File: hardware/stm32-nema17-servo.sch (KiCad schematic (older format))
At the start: 91 parts, among them J1 Conn_01x05, J2 C31-S-RA-CS1A-BK-SS, J3 TC-2050, J4 Screw_Terminal_01x02, J5 Screw_Terminal_01x02, J7 Conn_01x03, J8 Conn_01x03, J9 Conn_01x02, M1 Stepper_Motor_bipolar, Q1 NTTFS4937N, Q10 SSM3K35CTC, Q2 NVTFS5C658NL, Q3 NVTFS5C658NL, Q4 NVTFS5C658NL, Q5 NVTFS5C658NL, Q6 NVTFS5C658NL, Q7 NVTFS5C658NL, Q8 SSM3K35CTC, Q9 SSM3K35CTC, SW1 EVP-BB2A9B000, U1 STM32G431CBU, U2 74LVC2G32, U3 UCC27516, U4 AS5047D, U5 TPS62172DSG, U6 DRV8323RS

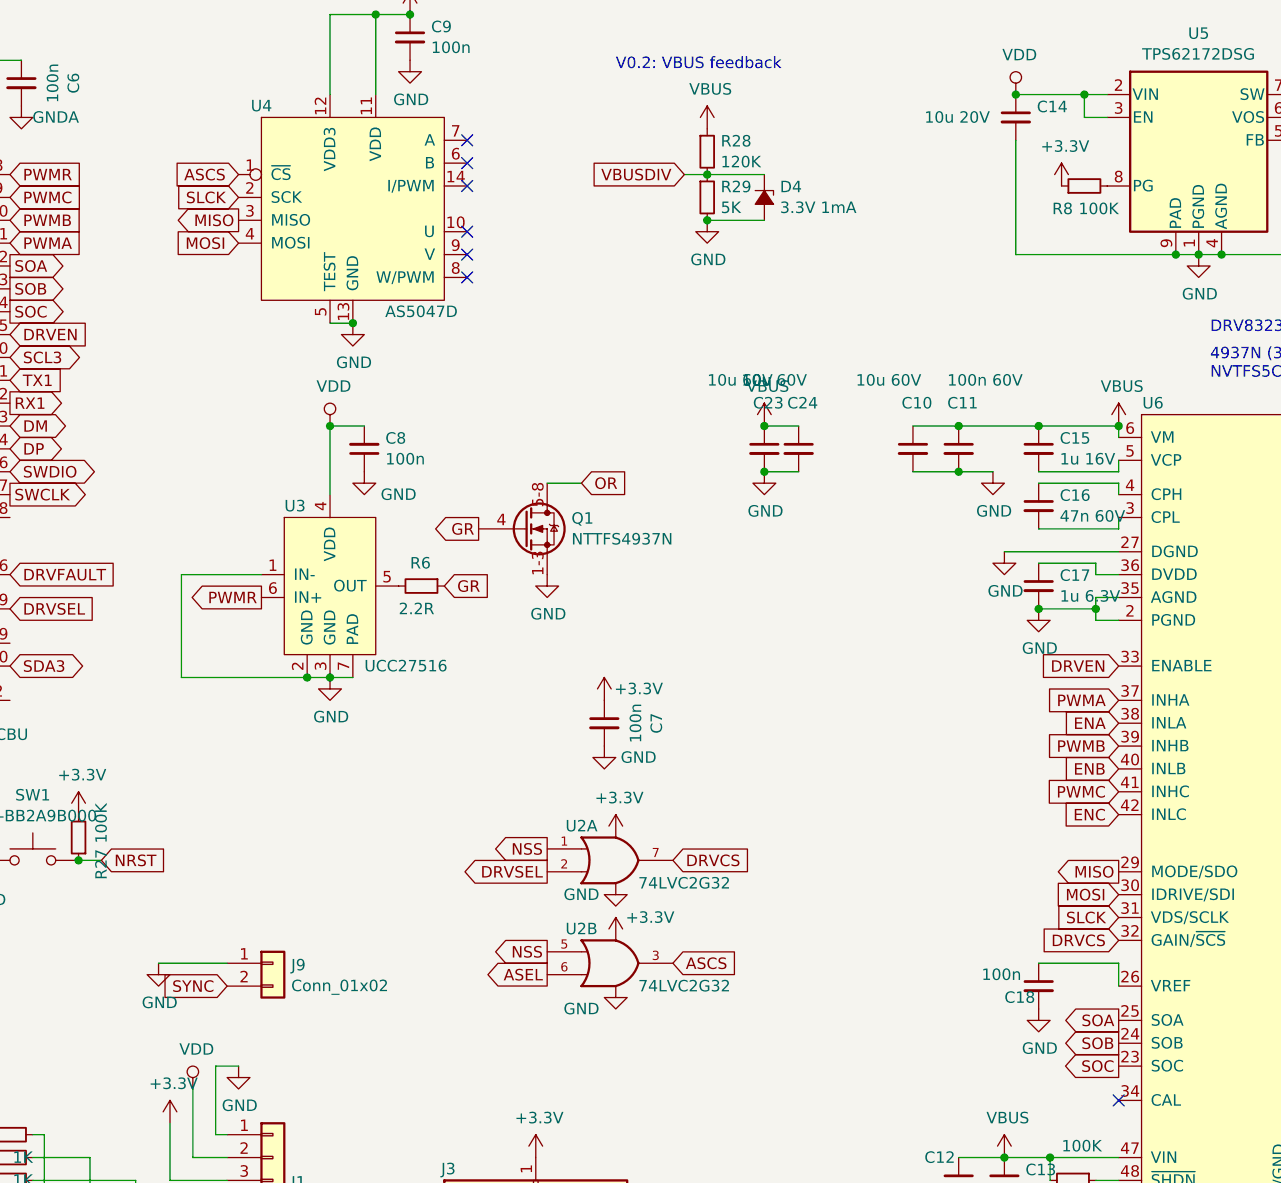
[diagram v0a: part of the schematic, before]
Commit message: further fixes on v0.2 hardware
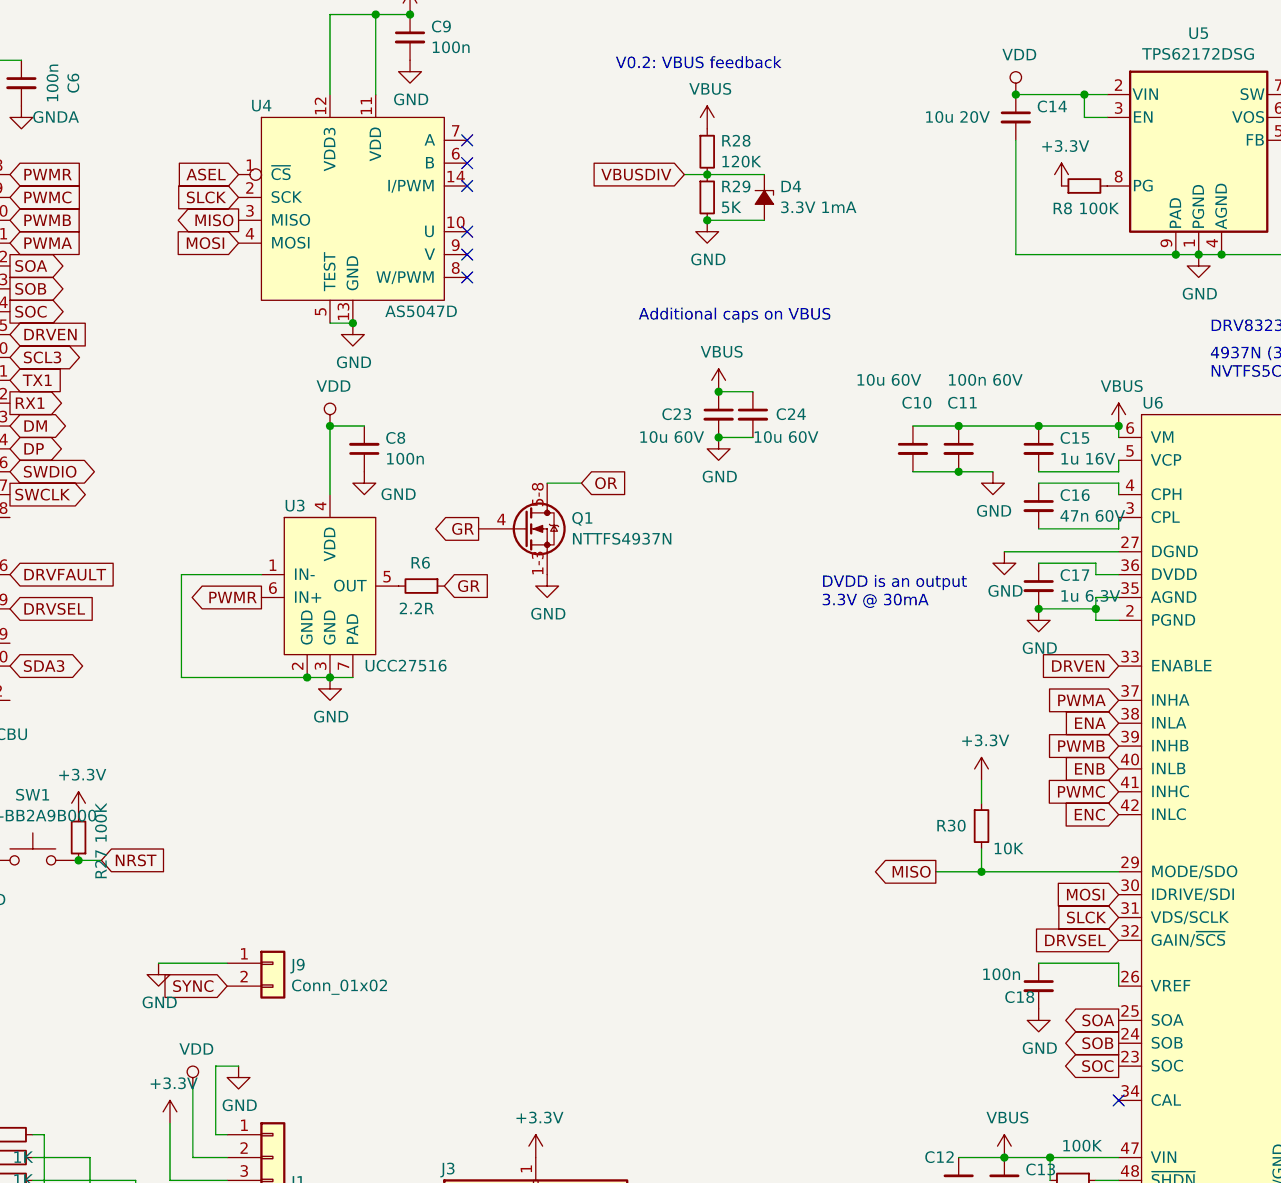
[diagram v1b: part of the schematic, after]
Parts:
- removed C7: 100n, Capacitor_SMD:C_0402_1005Metric, symbol Device:C_Small
- removed U2: 74LVC2G32, Package_SON:X2SON-8_1.4x1mm_P0.35mm, symbol 74xGxx:74LVC2G32
- added R30: 10K, Resistor_SMD:R_0402_1005Metric, symbol Device:R_Small
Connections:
- net ASCS is gone; now on net ASEL: U4.1 (~CS)
- net DRVCS is gone; now on net DRVSEL: U6.32 (GAIN/~SCS)
- net +3V3: now also R30.1
- net MISO: now also R30.2
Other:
- note added: "Additional caps on VBUS"
- note added: "DVDD is an output\n3.3V @ 30mA"
- moved on the sheet: C23, C24
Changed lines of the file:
@@
 Text GLabel 7450 4400 0    50   Input ~ 0
 ENC
-Text GLabel 7450 4650 0    50   Output ~ 0
+Text GLabel 6650 4650 0    50   Output ~ 0
 MISO
 Text GLabel 7450 4750 0    50   Input ~ 0
@@
 SLCK
 Text GLabel 7450 4950 0    50   Input ~ 0
-DRVCS
+DRVSEL
 Text GLabel 3600 1600 0    50   Input ~ 0
-ASCS
+ASEL
 Text GLabel 2600 1900 2    50   Input ~ 0
 PWMA
@@
 Text GLabel 1300 3700 0    50   Input ~ 0
 SLCK
-Text GLabel 5500 5050 2    50   Input ~ 0
-ASCS
-Text GLabel 5500 4600 2    50   Input ~ 0
-DRVCS
 Text GLabel 7450 5300 0    50   Output ~ 0
 SOA
@@
 	3150 6300 3550 6300
 Connection ~ 3150 6300
-Text GLabel 4950 4650 0    50   Output ~ 0
-DRVSEL
-Text GLabel 4950 5100 0    50   Output ~ 0
-ASEL
 Text GLabel 2600 3500 2    50   Input ~ 0
 DRVSEL
@@
 L Device:C_Small C23
 U 1 1 5D56448D
-P 5900 2800
-F 0 "C23" H 5850 3000 50  0000 L CNN
-F 1 "10u 60V" H 5650 3100 50  0000 L CNN
-F 2 "Capacitor_SMD:C_1210_3225Metric" H 5900 2800 50  0001 C CNN
-F 3 "~" H 5900 2800 50  0001 C CNN
-	1    5900 2800
+P 5700 2650
+F 0 "C23" H 5450 2650 50  0000 L CNN
+F 1 "10u 60V" H 5350 2550 50  0000 L CNN
+F 2 "Capacitor_SMD:C_1210_3225Metric" H 5700 2650 50  0001 C CNN
+F 3 "~" H 5700 2650 50  0001 C CNN
+	1    5700 2650
 	1    0    0    -1
 $EndComp
@@
 L power:VBUS #PWR059
 U 1 1 5D567754
-P 5900 2700
-F 0 "#PWR059" H 5900 2550 50  0001 C CNN
-F 1 "VBUS" H 5915 2873 50  0000 C CNN
-F 2 "" H 5900 2700 50  0001 C CNN
-F 3 "" H 5900 2700 50  0001 C CNN
-	1    5900 2700
+P 5700 2550
+F 0 "#PWR059" H 5700 2400 50  0001 C CNN
+F 1 "VBUS" H 5715 2723 50  0000 C CNN
+F 2 "" H 5700 2550 50  0001 C CNN
+F 3 "" H 5700 2550 50  0001 C CNN
+	1    5700 2550
 	1    0    0    -1
 $EndComp
@@
 L power:GND #PWR060
 U 1 1 5D56F0C9
-P 5900 2900
-F 0 "#PWR060" H 5900 2650 50  0001 C CNN
-F 1 "GND" H 5905 2727 50  0000 C CNN
-F 2 "" H 5900 2900 50  0001 C CNN
-F 3 "" H 5900 2900 50  0001 C CNN
-	1    5900 2900
+P 5700 2750
+F 0 "#PWR060" H 5700 2500 50  0001 C CNN
+F 1 "GND" H 5705 2577 50  0000 C CNN
+F 2 "" H 5700 2750 50  0001 C CNN
+F 3 "" H 5700 2750 50  0001 C CNN
+	1    5700 2750
 	1    0    0    -1
 $EndComp
@@
 L Device:C_Small C24
 U 1 1 5D57E91C
-P 6050 2800
-F 0 "C24" H 6000 3000 50  0000 L CNN
-F 1 "10u 60V" H 5800 3100 50  0000 L CNN
-F 2 "Capacitor_SMD:C_1210_3225Metric" H 6050 2800 50  0001 C CNN
-F 3 "~" H 6050 2800 50  0001 C CNN
-	1    6050 2800
-	1    0    0    -1
-$EndComp
-Wire Wire Line
-	5900 2700 6050 2700
-Connection ~ 5900 2700
-Wire Wire Line
-	6050 2900 5900 2900
-Connection ~ 5900 2900
+P 5850 2650
+F 0 "C24" H 5950 2650 50  0000 L CNN
+F 1 "10u 60V" H 5850 2550 50  0000 L CNN
+F 2 "Capacitor_SMD:C_1210_3225Metric" H 5850 2650 50  0001 C CNN
+F 3 "~" H 5850 2650 50  0001 C CNN
+	1    5850 2650
+	1    0    0    -1
+$EndComp
+Wire Wire Line
+	5700 2550 5850 2550
+Connection ~ 5700 2550
+Wire Wire Line
+	5850 2750 5700 2750
+Connection ~ 5700 2750
 $Comp
 L Switch:SW_Push SW1
@@
 Text Notes 5250 1150 0    50   ~ 0
 V0.2: VBUS feedback
-$Comp
-L power:GND #PWR017
-U 1 1 5D97ADCA
-P 5200 4100
-F 0 "#PWR017" H 5200 3850 50  0001 C CNN
-F 1 "GND" H 5350 4050 50  0000 C CNN
-F 2 "" H 5200 4100 50  0001 C CNN
-F 3 "" H 5200 4100 50  0001 C CNN
-	1    5200 4100
+Text Notes 6150 3500 0    50   ~ 0
+DVDD is an output\n3.3V @ 30mA
+Text Notes 5350 2250 0    50   ~ 0
+Additional caps on VBUS
+$Comp
+L Device:R_Small R30
+U 1 1 5D7DCDEC
+P 6850 4450
+F 0 "R30" H 6650 4450 50  0000 L CNN
+F 1 "10K" H 6900 4350 50  0000 L CNN
+F 2 "Resistor_SMD:R_0402_1005Metric" H 6850 4450 50  0001 C CNN
+F 3 "~" H 6850 4450 50  0001 C CNN
+	1    6850 4450
 	1    0    0    -1
 $EndComp
 $Comp
 L power:+3.3V #PWR016
-U 1 1 5D97AAED
-P 5200 3900
-F 0 "#PWR016" H 5200 3750 50  0001 C CNN
-F 1 "+3.3V" H 5350 3950 50  0000 C CNN
-F 2 "" H 5200 3900 50  0001 C CNN
-F 3 "" H 5200 3900 50  0001 C CNN
-	1    5200 3900
-	1    0    0    -1
-$EndComp
-$Comp
-L Device:C_Small C7
-U 1 1 5D97A3CE
-P 5200 4000
-F 0 "C7" V 5429 4000 50  0000 C CNN
-F 1 "100n" V 5338 4000 50  0000 C CNN
-F 2 "Capacitor_SMD:C_0402_1005Metric" H 5200 4000 50  0001 C CNN
-F 3 "~" H 5200 4000 50  0001 C CNN
-	1    5200 4000
-	1    0    0    -1
-$EndComp
-$Comp
-L power:GND #PWR019
-U 1 1 5D9438D7
-P 5250 4700
-F 0 "#PWR019" H 5250 4450 50  0001 C CNN
-F 1 "GND" H 5100 4650 50  0000 C CNN
-F 2 "" H 5250 4700 50  0001 C CNN
-F 3 "" H 5250 4700 50  0001 C CNN
-	1    5250 4700
-	1    0    0    -1
-$EndComp
-$Comp
-L power:GND #PWR021
-U 1 1 5D9435E1
-P 5250 5150
-F 0 "#PWR021" H 5250 4900 50  0001 C CNN
-F 1 "GND" H 5100 5050 50  0000 C CNN
-F 2 "" H 5250 5150 50  0001 C CNN
-F 3 "" H 5250 5150 50  0001 C CNN
-	1    5250 5150
-	1    0    0    -1
-$EndComp
-$Comp
-L power:+3.3V #PWR020
-U 1 1 5D943303
-P 5250 4950
-F 0 "#PWR020" H 5250 4800 50  0001 C CNN
-F 1 "+3.3V" H 5400 5050 50  0000 C CNN
-F 2 "" H 5250 4950 50  0001 C CNN
-F 3 "" H 5250 4950 50  0001 C CNN
-	1    5250 4950
-	1    0    0    -1
-$EndComp
-$Comp
-L power:+3.3V #PWR018
-U 1 1 5D9428FC
-P 5250 4500
-F 0 "#PWR018" H 5250 4350 50  0001 C CNN
-F 1 "+3.3V" H 5265 4673 50  0000 C CNN
-F 2 "" H 5250 4500 50  0001 C CNN
-F 3 "" H 5250 4500 50  0001 C CNN
-	1    5250 4500
-	1    0    0    -1
-$EndComp
-Text GLabel 4950 4550 0    50   Output ~ 0
-NSS
-Text GLabel 4950 5000 0    50   Output ~ 0
-NSS
-$Comp
-L 74xGxx:74LVC2G32 U2
-U 2 1 5D936E11
-P 5250 5050
-F 0 "U2" H 5100 5200 50  0000 C CNN
-F 1 "74LVC2G32" H 5550 4950 50  0000 C CNN
-F 2 "Package_SON:X2SON-8_1.4x1mm_P0.35mm" H 5250 5050 50  0001 C CNN
-F 3 "http://www.ti.com/lit/sg/scyt129e/scyt129e.pdf" H 5250 5050 50  0001 C CNN
-	2    5250 5050
-	1    0    0    -1
-$EndComp
-$Comp
-L 74xGxx:74LVC2G32 U2
-U 1 1 5D935F70
-P 5250 4600
-F 0 "U2" H 5100 4750 50  0000 C CNN
-F 1 "74LVC2G32" H 5550 4500 50  0000 C CNN
-F 2 "Package_SON:X2SON-8_1.4x1mm_P0.35mm" H 5250 4600 50  0001 C CNN
-F 3 "http://www.ti.com/lit/sg/scyt129e/scyt129e.pdf" H 5250 4600 50  0001 C CNN
-	1    5250 4600
-	1    0    0    -1
-$EndComp
+U 1 1 5D7EA92E
+P 6850 4250
+F 0 "#PWR016" H 6850 4100 50  0001 C CNN
+F 1 "+3.3V" H 6865 4423 50  0000 C CNN
+F 2 "" H 6850 4250 50  0001 C CNN
+F 3 "" H 6850 4250 50  0001 C CNN
+	1    6850 4250
+	1    0    0    -1
+$EndComp
+Wire Wire Line
+	6850 4250 6850 4350
+Wire Wire Line
+	6650 4650 6850 4650
+Wire Wire Line
+	6850 4550 6850 4650
+Connection ~ 6850 4650
+Wire Wire Line
+	6850 4650 7450 4650
 $EndSCHEMATC
